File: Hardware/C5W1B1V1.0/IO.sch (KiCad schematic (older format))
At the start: 3 parts, among them J1 Conn_02x20_Counter_Clockwise, J2 Conn_02x20_Counter_Clockwise, J4 Conn_01x04

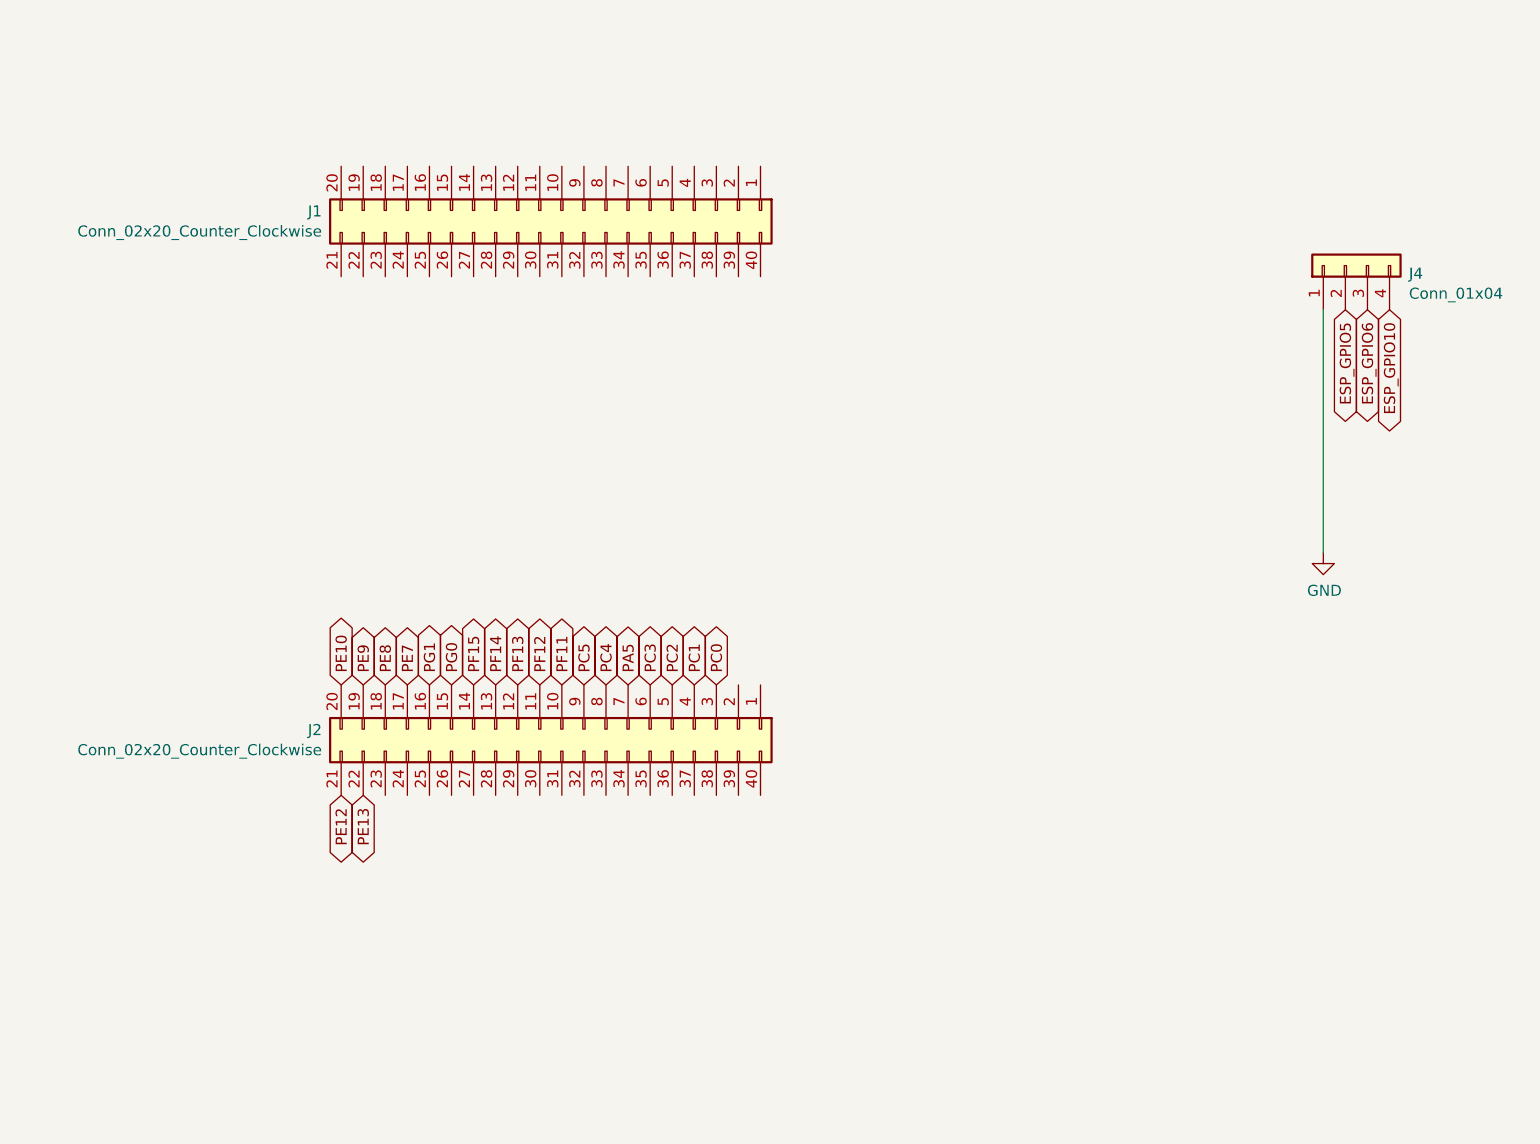
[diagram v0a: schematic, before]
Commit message: Rozlana masa
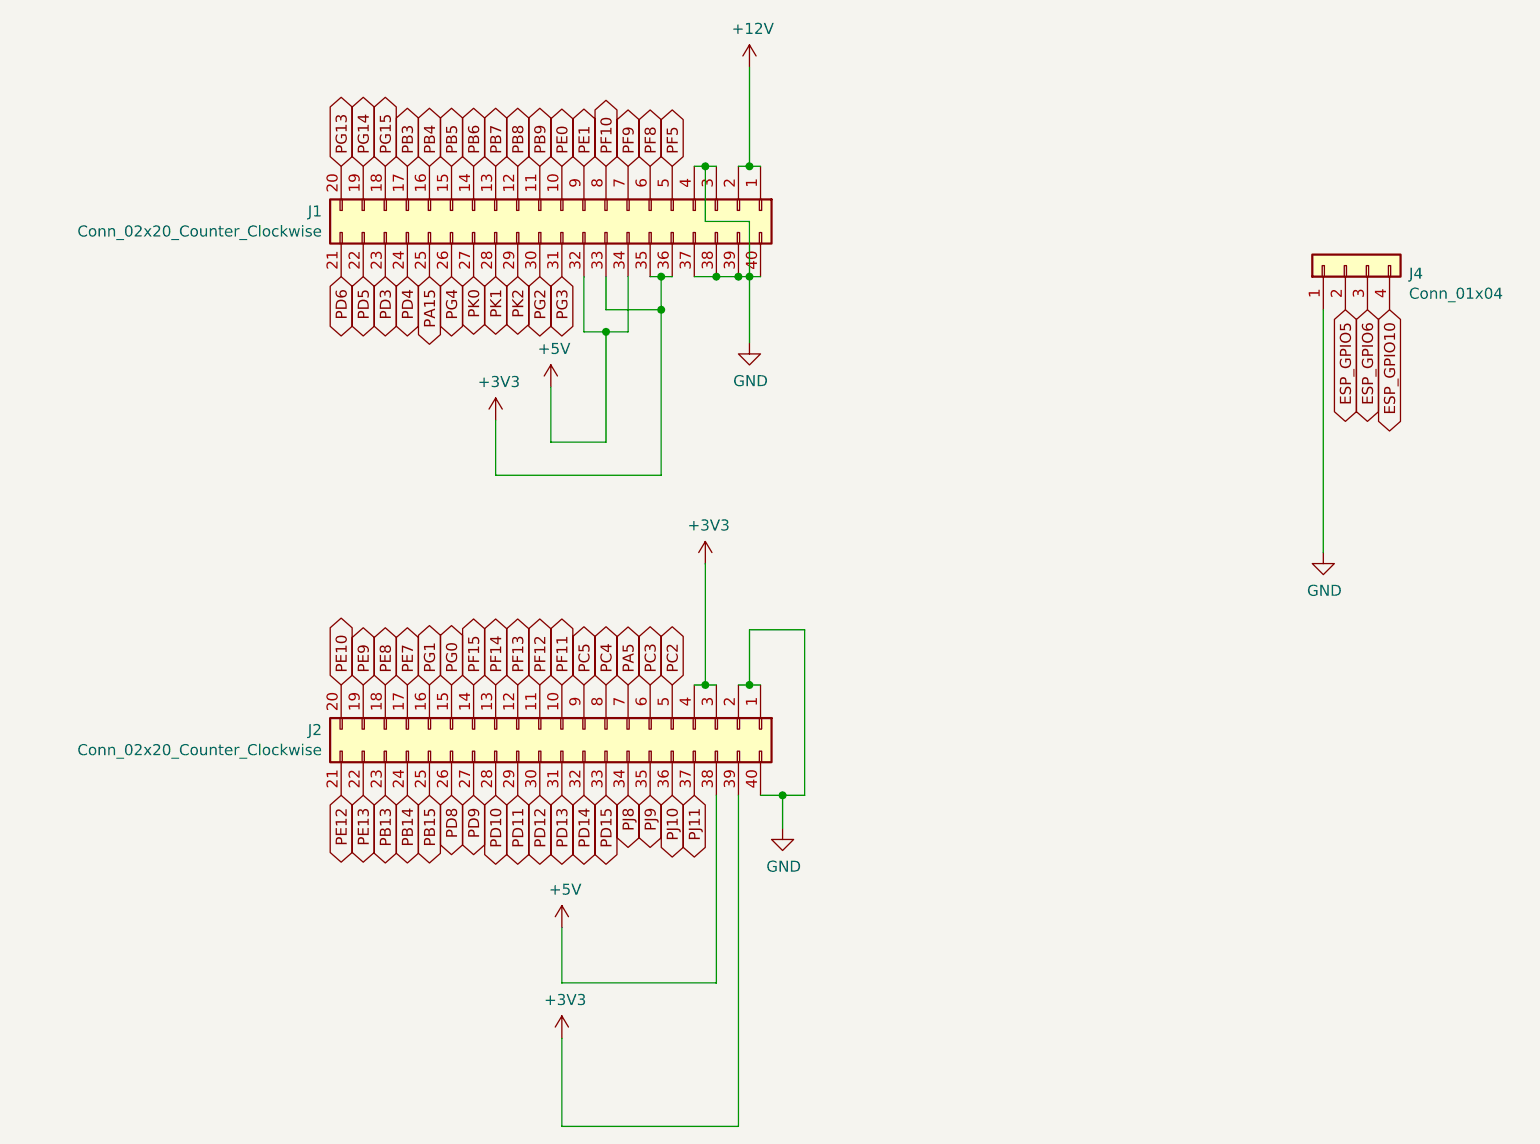
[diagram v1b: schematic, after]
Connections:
- net PC0 is gone; now on net +3V3: J2.3 (Pin_3)
- net PC1 is gone; now on net +3V3: J2.4 (Pin_4)
- net GND: now also J1.3 (Pin_3), J1.37 (Pin_37), J1.38 (Pin_38), J1.39 (Pin_39), J1.4 (Pin_4), J1.40 (Pin_40), J2.1 (Pin_1), J2.2 (Pin_2), J2.40 (Pin_40)
- net +12V: now reaches J1.1 (Pin_1)
- net +12V: now also J1.2 (Pin_2)
- net PE0: now reaches J1.10 (Pin_10)
- net PB9: now reaches J1.11 (Pin_11)
- net PB8: now reaches J1.12 (Pin_12)
- net PB7: now reaches J1.13 (Pin_13)
- net PB6: now reaches J1.14 (Pin_14)
- net PB5: now reaches J1.15 (Pin_15)
- net PB4: now reaches J1.16 (Pin_16)
- net PB3: now reaches J1.17 (Pin_17)
- net PG15: now reaches J1.18 (Pin_18)
- net PG14: now reaches J1.19 (Pin_19)
- net PG13: now reaches J1.20 (Pin_20)
- net PD6: now reaches J1.21 (Pin_21)
- net PD5: now reaches J1.22 (Pin_22)
- net PD3: now reaches J1.23 (Pin_23)
- net PD4: now reaches J1.24 (Pin_24)
- net PA15: now reaches J1.25 (Pin_25)
- net PG4: now reaches J1.26 (Pin_26)
- net PK0: now reaches J1.27 (Pin_27)
- net PK1: now reaches J1.28 (Pin_28)
- net PK2: now reaches J1.29 (Pin_29)
- net PG2: now reaches J1.30 (Pin_30)
- net PG3: now reaches J1.31 (Pin_31)
- net +5V: now reaches J1.32 (Pin_32)
- net +5V: now also J1.34 (Pin_34), J2.38 (Pin_38)
- net +3V3: now reaches J1.33 (Pin_33)
- net +3V3: now also J1.35 (Pin_35), J1.36 (Pin_36), J2.39 (Pin_39)
- net PF5: now reaches J1.5 (Pin_5)
- net PF8: now reaches J1.6 (Pin_6)
- net PF9: now reaches J1.7 (Pin_7)
- net PF10: now reaches J1.8 (Pin_8)
- net PE1: now reaches J1.9 (Pin_9)
- net PB13: now reaches J2.23 (Pin_23)
- net PB14: now reaches J2.24 (Pin_24)
- net PB15: now reaches J2.25 (Pin_25)
- net PD8: now reaches J2.26 (Pin_26)
- net PD9: now reaches J2.27 (Pin_27)
- net PD10: now reaches J2.28 (Pin_28)
- net PD11: now reaches J2.29 (Pin_29)
- net PD12: now reaches J2.30 (Pin_30)
- net PD13: now reaches J2.31 (Pin_31)
- net PD14: now reaches J2.32 (Pin_32)
- net PD15: now reaches J2.33 (Pin_33)
- net PJ8: now reaches J2.34 (Pin_34)
- net PJ9: now reaches J2.35 (Pin_35)
- net PJ10: now reaches J2.36 (Pin_36)
- net PJ11: now reaches J2.37 (Pin_37)
